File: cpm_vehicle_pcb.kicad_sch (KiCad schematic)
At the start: 88 parts, among them IC1 ATMEGAAU, IC2 RPI-ZERO, J1 Conn_02x03_Counter_Clockwise, J2 Conn_02x03_Counter_Clockwise, J3 Conn_01x05, J4 USB4105-GF-A, J5 USB_B_Mini, J6 Conn_01x03_Socket, J7 USB4105-GF-A, P1 NCP1117, Q11 BSS123, Q12 BSS123, Q13 BSS123, Q14 BSS123, Q3 DMG9926UDM, SW1 SW_DIP_x02, SW2 SW_SPDT_312, U1 BQ25887RGET, U3 TXB0104PWR, U4 MT3608, U7 CH340G, U8 R5460N

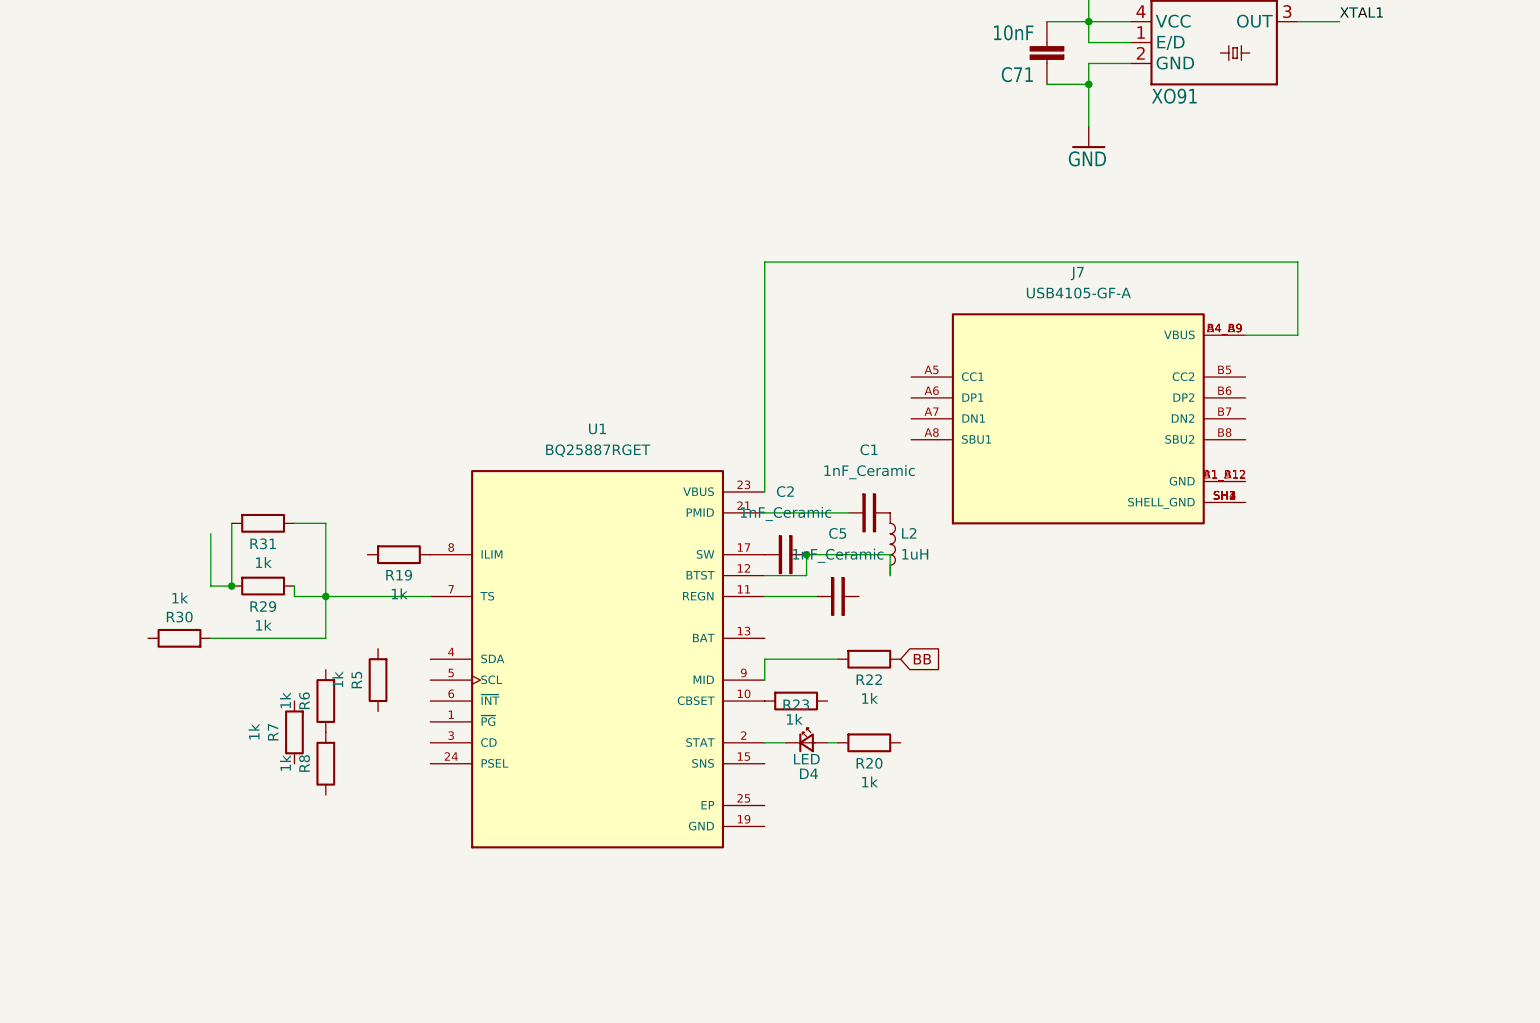
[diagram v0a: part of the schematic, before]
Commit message: Schematic BQ25887
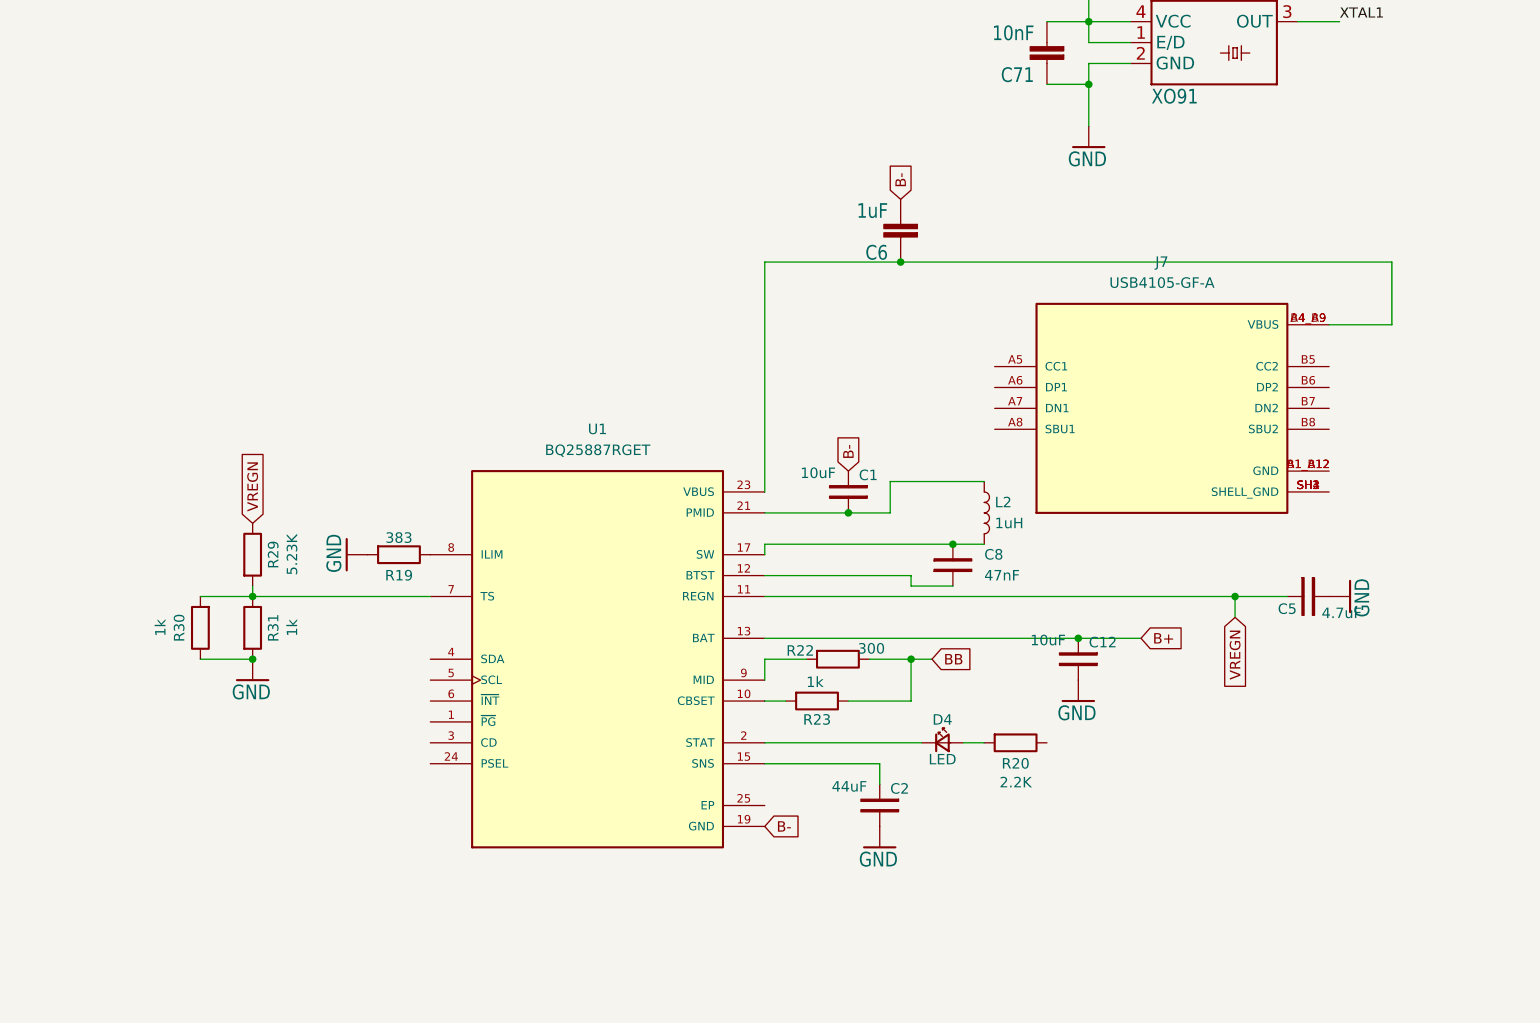
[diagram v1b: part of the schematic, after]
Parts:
- removed R5, R6, R7, R8: 1k, Resistor_SMD:R_0603_1608Metric, symbol Device:R
- added C12: 10uF, Capacitor_THT:C_Disc_D5.0mm_W2.5mm_P2.50mm, symbol PCM_SL_Capacitors:1nF_Ceramic
- added C6: 1uF, footprints_vehicle_pcb:C0805_10681391, symbol main_board_V2.4-eagle-import:embedded_10681391_C-EUC0805
- added C8: 47nF, Capacitor_THT:C_Disc_D5.0mm_W2.5mm_P2.50mm, symbol PCM_SL_Capacitors:1nF_Ceramic
- C1: value 1nF_Ceramic -> 10uF
- C2: value 1nF_Ceramic -> 44uF
- C5: value 1nF_Ceramic -> 4.7uF
- R19: value 1k -> 383
- R20: value 1k -> 2.2K
- R22: value 1k -> 300
- R29: value 1k -> 5.23K
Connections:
- net B+ is gone; now on net BAT: J6.3 (Pin_3), R25.1, SW2.1 (B)
- net B- is gone; now on net GND: C11.2, C9.2, J6.1 (Pin_1), Q3.3 (S2), U8.6 (VSS)
- net BAT: now also C12.1
- net BB: now also R23.1
- net GND: now also C1.1, C2.2, C5.2, R19.2, R30.1, R31.2, C12.2, C6.2
- net PMID: now also C1.2, L2.1; no longer C1.1
- net SW: now also L2.2, C8.2; no longer C2.1
- net at R30.2, R31.1, U1.7 (TS): now also R29.2; no longer R29.1
- net VREGN: now reaches C5.1, U1.11 (REGN)
- net VREGN: now also R29.1
- net at J7.A4_B9 (VBUS), J7.B4_A9 (VBUS), U1.23 (VBUS): now also C6.1
- net at U1.15 (SNS), U1.16 (SNS): now also C2.1
- new net: C8.1, U1.12 (BTST)
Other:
- moved on the sheet: C1, C5, D4, J7, L2, R20, R22, R23, R29, R30, R31
